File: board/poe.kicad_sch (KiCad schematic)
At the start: 5 parts, among them J2 SS-73100-082, J3 SS-73100-082, J5 768250002

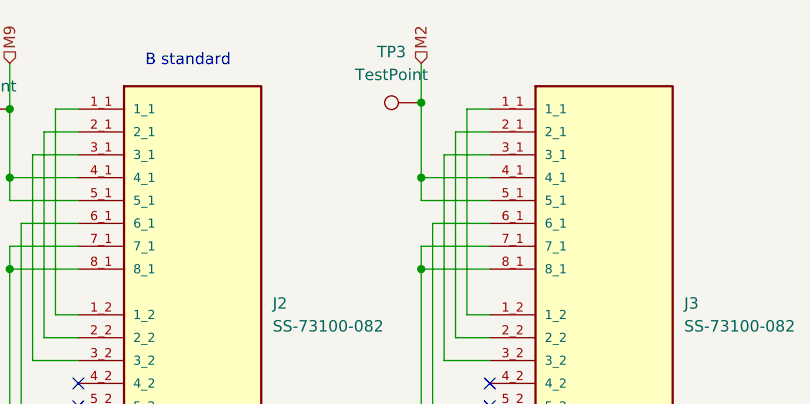
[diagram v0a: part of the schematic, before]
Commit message: 17 hours of our lives
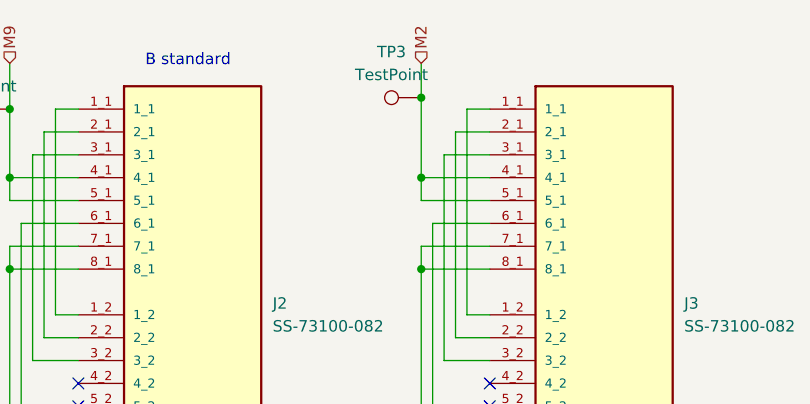
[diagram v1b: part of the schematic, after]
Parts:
- TP2, TP3: footprint Connector_Pin:Pin_D1.1mm_L10.2mm_W3.5mm_Flat -> TestPoint:TestPoint_Pad_D1.0mm
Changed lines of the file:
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@@
-	)
-	(junction
-		(at 83.82 38.6595)
-		(diameter 0)
-		(color 0 0 0 0)
 	)
 	(junction
@@
 	)
 	(junction
+		(at 83.82 38.1)
+		(diameter 0)
+		(color 0 0 0 0)
+	)
+	(junction
 		(at 83.82 85.09)
 		(diameter 0)
@@
 	(wire
 		(pts
-			(xy 83.82 38.6595) (xy 83.82 46.99)
+			(xy 83.82 34.29) (xy 83.82 38.1)
 		)
 		(stroke
@@
 	(wire
 		(pts
+			(xy 83.82 38.1) (xy 83.82 46.99)
+		)
+		(stroke
+			(width 0)
+			(type default)
+		)
+	)
+	(wire
+		(pts
 			(xy 85.09 52.07) (xy 85.09 74.93)
 		)
@@
 		(pts
 			(xy 45.72 85.09) (xy 38.1 85.09)
-		)
-		(stroke
-			(width 0)
-			(type default)
-		)
-	)
-	(wire
-		(pts
-			(xy 83.82 34.29) (xy 83.82 38.6595)
 		)
 		(stroke
@@
 			)
 		)
-		(property "Footprint" "Connector_Pin:Pin_D1.1mm_L10.2mm_W3.5mm_Flat"
+		(property "Footprint" "TestPoint:TestPoint_Pad_D1.0mm"
 			(at 38.1 34.29 0)
 			(effects
@@
 	)
 	(symbol
+		(lib_id "Connector:TestPoint")
+		(at 83.82 38.1 90)
+		(unit 1)
+		(exclude_from_sim no)
+		(in_bom yes)
+		(on_board yes)
+		(dnp no)
+		(fields_autoplaced yes)
+		(property "Reference" "TP3"
+			(at 80.518 33.02 90)
+			(effects
+				(font
+					(size 1.27 1.27)
+				)
+			)
+		)
+		(property "Value" "TestPoint"
+			(at 80.518 35.56 90)
+			(effects
+				(font
+					(size 1.27 1.27)
+				)
+			)
+		)
+		(property "Footprint" "TestPoint:TestPoint_Pad_D1.0mm"
+			(at 83.82 33.02 0)
+			(effects
+				(font
+					(size 1.27 1.27)
+				)
+				(hide yes)
+			)
+		)
+		(property "Datasheet" "~"
+			(at 83.82 33.02 0)
+			(effects
+				(font
+					(size 1.27 1.27)
+				)
+				(hide yes)
+			)
+		)
+		(property "Description" "test point"
+			(at 83.82 38.1 0)
+			(effects
+				(font
+					(size 1.27 1.27)
+				)
+				(hide yes)
+			)
+		)
+		(pin "1"
+		)
+		(instances
+			(project "PowerManagementBoard"
+				(path "/7eaa639d-7062-45e7-be05-1c2855431307/a330d3b6-4e53-4d10-a34b-46d7b687198c"
+					(reference "TP3")
+					(unit 1)
+				)
+			)
+		)
+	)
+	(symbol
 		(lib_id "PowerManagementBoard:768250002")
 		(at 34.29 119.38 180)
@@
 					(unit 1)
 				)
-			)
-		)
-	)
-	(symbol
-		(lib_id "Connector:TestPoint")
-		(at 83.82 38.6595 90)
-		(unit 1)
-		(exclude_from_sim no)
-		(in_bom yes)
-		(on_board yes)
-		(dnp no)
-		(fields_autoplaced yes)
-		(property "Reference" "TP3"
-			(at 80.518 33.02 90)
-			(effects
-				(font
-					(size 1.27 1.27)
-				)
-			)
-		)
-		(property "Value" "TestPoint"
-			(at 80.518 35.56 90)
-			(effects
-				(font
-					(size 1.27 1.27)
-				)
-			)
-		)
-		(property "Footprint" "Connector_Pin:Pin_D1.1mm_L10.2mm_W3.5mm_Flat"
-			(at 83.82 33.5795 0)
-			(effects
-				(font
-					(size 1.27 1.27)
-				)
-				(hide yes)
-			)
-		)
-		(property "Datasheet" "~"
-			(at 83.82 33.5795 0)
-			(effects
-				(font
-					(size 1.27 1.27)
-				)
-				(hide yes)
-			)
-		)
-		(property "Description" "test point"
-			(at 83.82 38.6595 0)
-			(effects
-				(font
-					(size 1.27 1.27)
-				)
-				(hide yes)
-			)
-		)
-		(pin "1"
-		)
-		(instances
-			(project "PowerManagementBoard"
-				(path "/7eaa639d-7062-45e7-be05-1c2855431307/a330d3b6-4e53-4d10-a34b-46d7b687198c"
-					(reference "TP3")
-					(unit 1)
-				)
